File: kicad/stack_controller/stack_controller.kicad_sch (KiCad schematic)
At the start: 46 parts

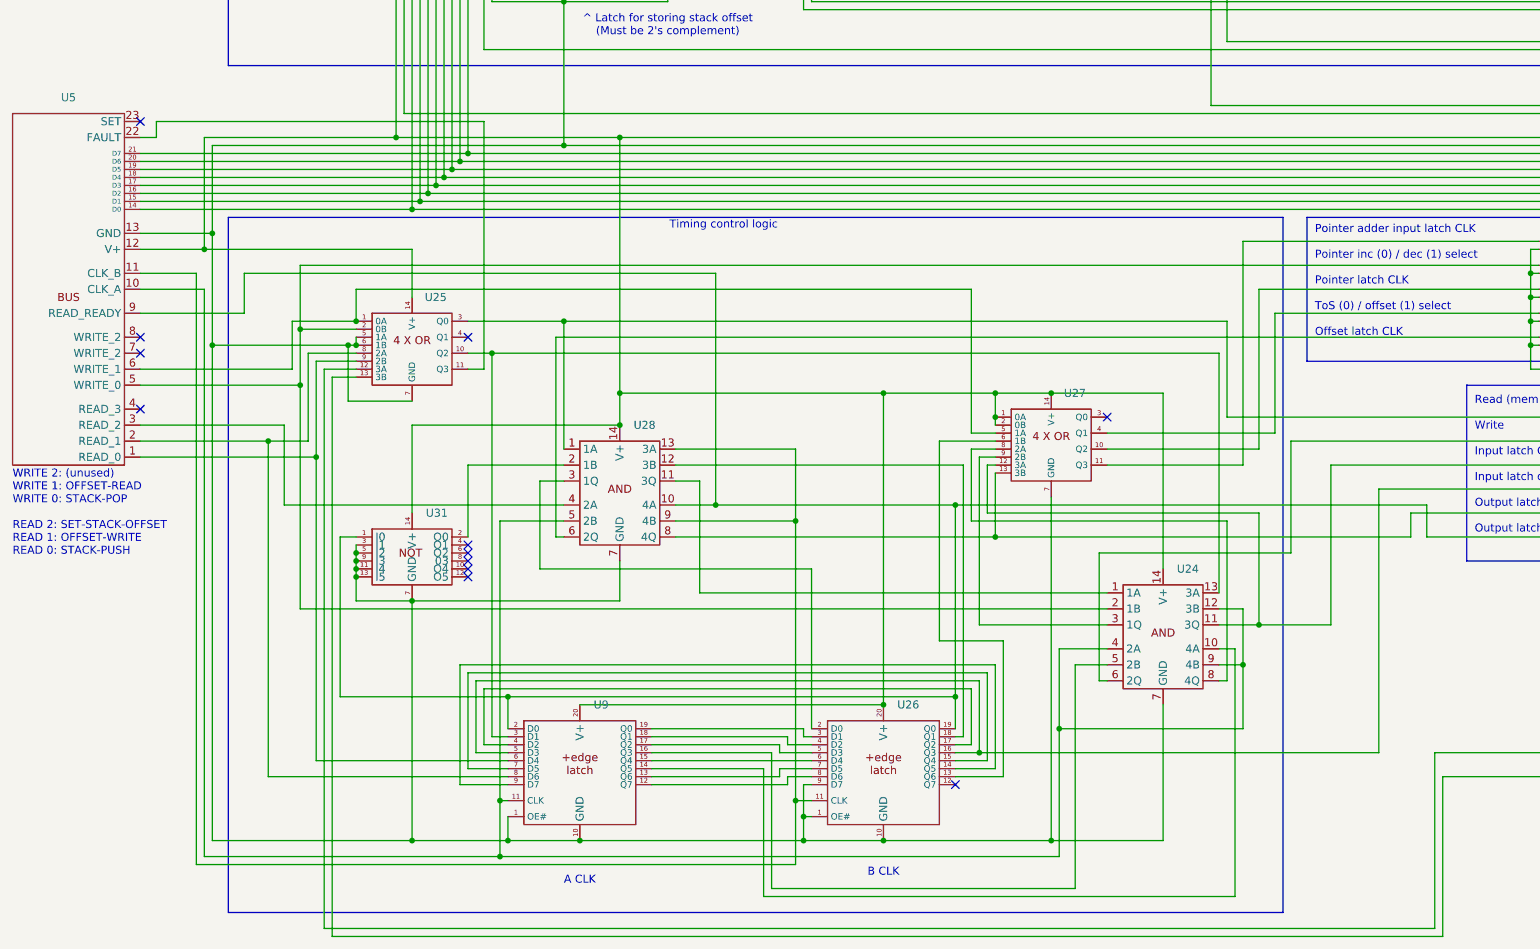
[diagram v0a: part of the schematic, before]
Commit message: stuff
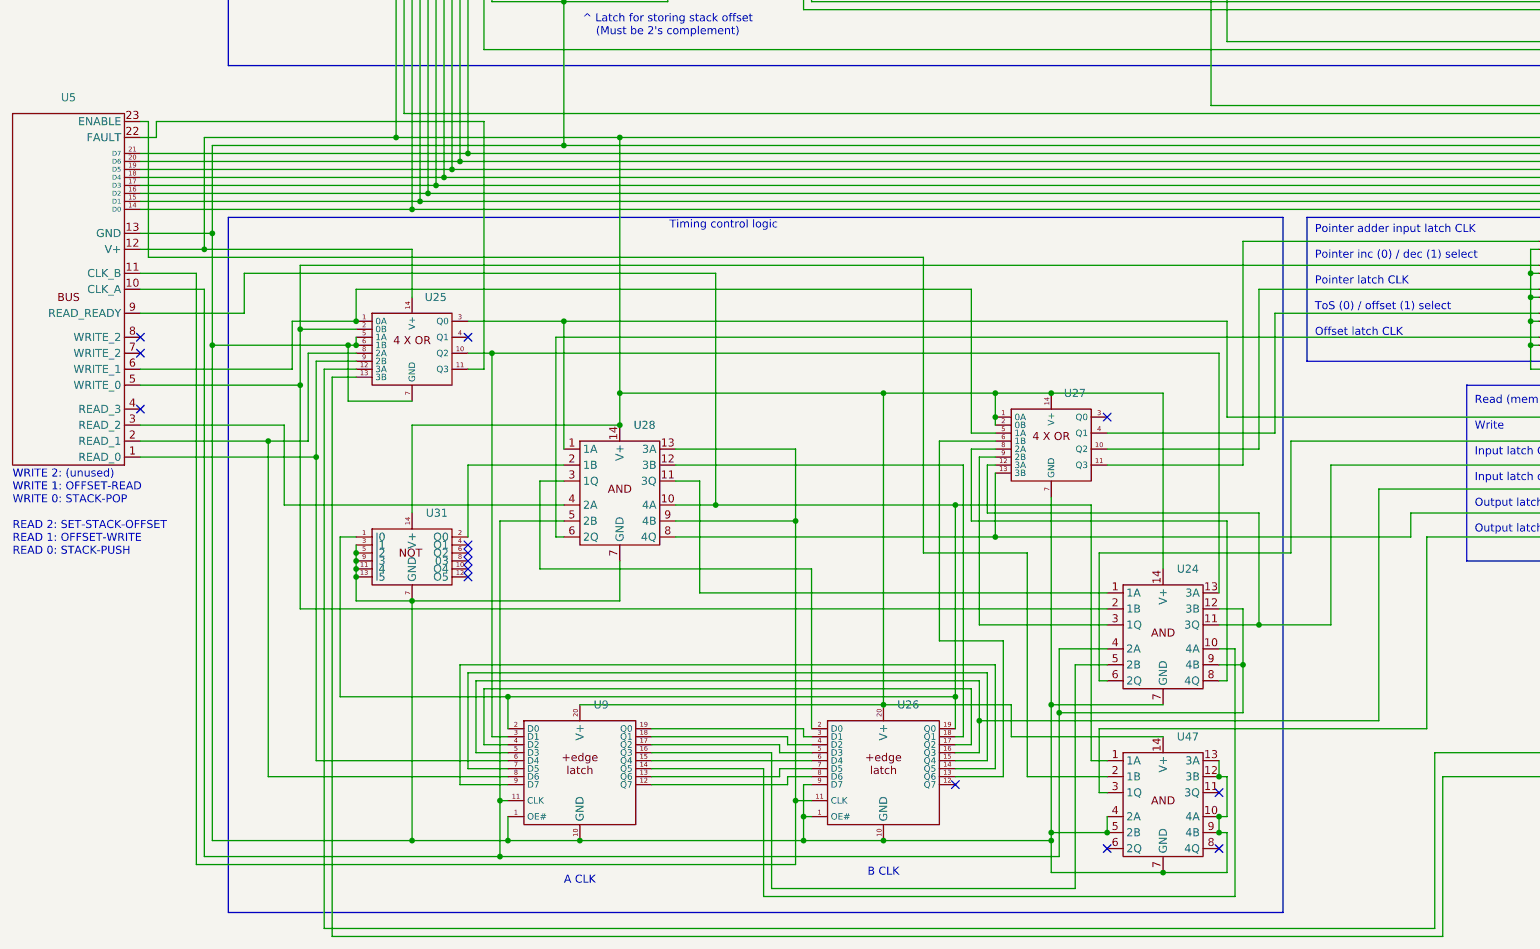
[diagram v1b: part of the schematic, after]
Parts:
- added U47: ~, Package_DIP:DIP-14_W7.62mm, symbol custom_symbol_lib:quad_and
- U1, U10, U11, U12, U13, U14, U15, U16, U17, U18, U19, U2, U20, U21, U22, U23, U24, U25, U26, U27, U28, U29, U3, U30, U31, U32, U33, U34, U35, U36, U37, U38, U39, U4, U40, U41, U42, U43, U44, U45, U46, U5, U6, U7, U8, U9: value (none) -> ~
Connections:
- net at U1.7 (C_IN), U1.8 (GND), U10.14 (GND)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: now also U47.10 (4A), U47.12 (3B), U47.13 (3A), U47.4 (2A), U47.5 (2B), U47.7 (GND), U47.9 (4B)
- net at U1.16 (V+), U1.6 (B0), U10.28 (V+)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: now also U47.14 (V+)
- net at U5.23 (ENABLE): now also U47.2 (1B)
- net at U26.19 (Q0), U28.10 (4A), U31.1 (I0)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: now also U47.1 (1A); no longer U44.1 (IN)
- new net: U44.1 (IN), U47.3 (1Q)
- no-connect marks 14 -> 16
